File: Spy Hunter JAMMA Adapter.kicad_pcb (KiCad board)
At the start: 2 copper layers, 111.4 x 135.4 mm, 88 parts, among them P1 1K, P2 1K, P3 10K, P4 1K, SW2 SW_DIP_SPSTx02_Slide_9.78x7.2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, U1 74LS86, U10 NE555, U11 LM386, U12 CD4099B, U2 74LS74, U3 74LS00, U4 74LS00, U5 74LS191, U6 74LS191, U7 NE555, U8 74LS157, U9 74LS157

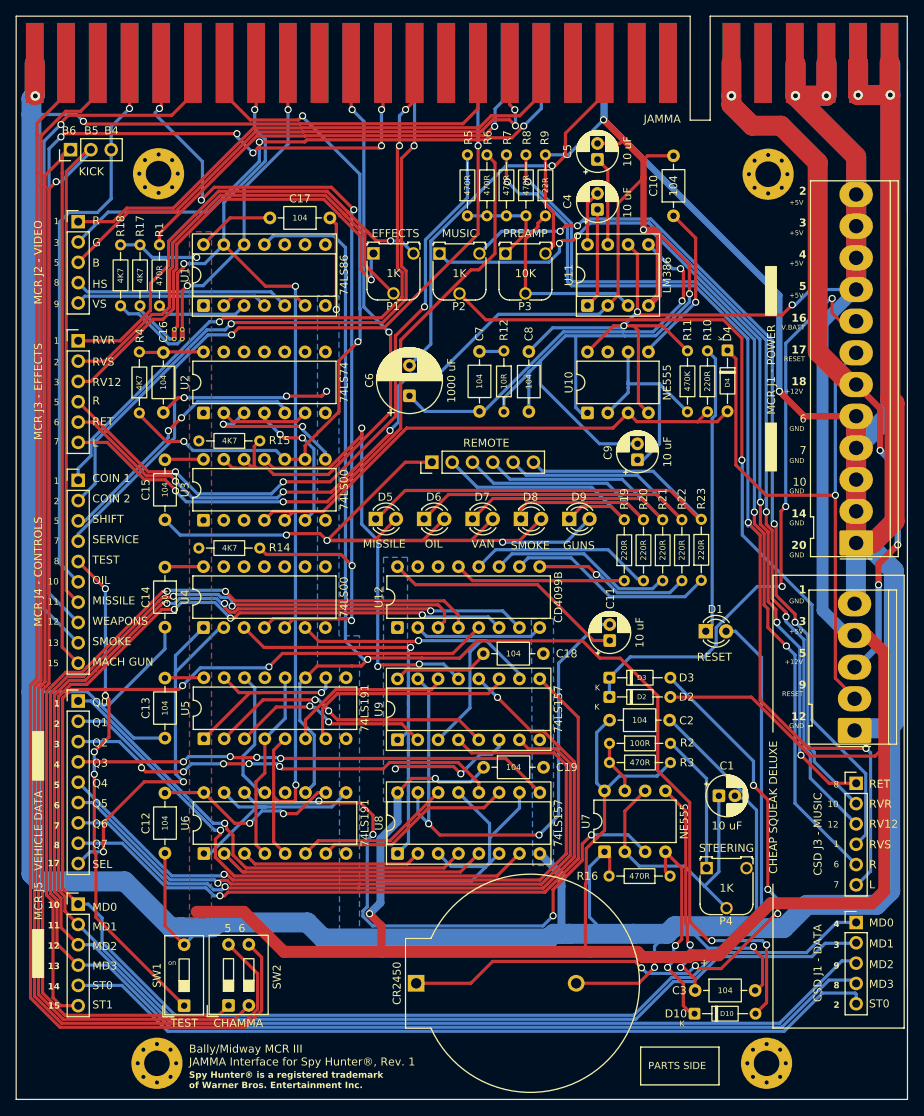
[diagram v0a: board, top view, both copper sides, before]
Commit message: minor cleanup and fine tuning
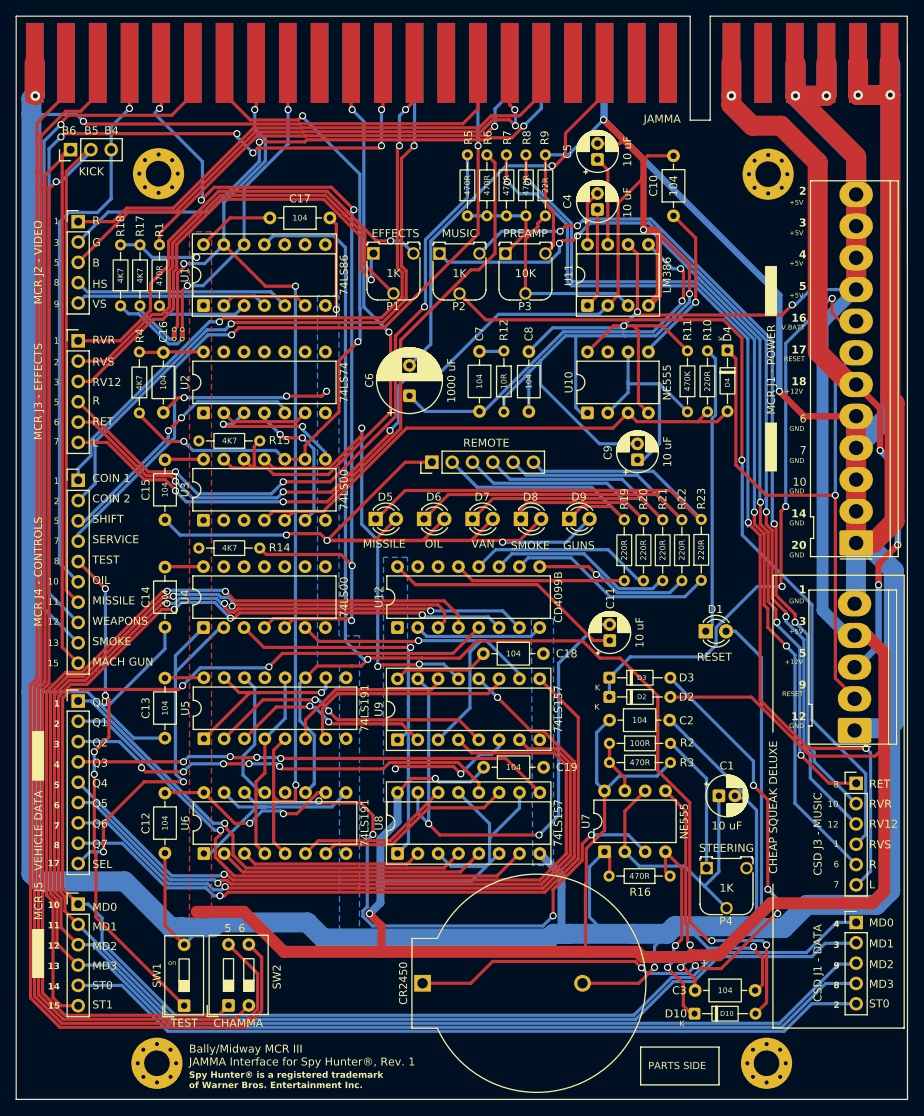
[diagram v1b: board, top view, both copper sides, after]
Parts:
- moved CR2450 0.80 mm to (105.2, 147.4)
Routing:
- net J5_ST0: track 102.9 -> 101.0 mm
- net EFFECTS_RVR: track 57.8 -> 56.6 mm
- net BATT+: track 85.3 -> 84.5 mm
- net GND: track 1352.2 -> 1351.4 mm
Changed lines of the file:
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@@
 		(tags "Resistor Axial_DIN0204 series Axial Horizontal pin pitch 7.62mm 0.167W length 3.6mm diameter 1.6mm")
 		(property "Reference" "R16"
-			(at 10.335 0 0)
+			(at 3.735 -2 0)
 			(layer "F.SilkS")
 			(effects
@@
 	(footprint "Battery:BatteryHolder_ComfortableElectronic_CH273-2450_1x2450"
 		(layer "F.Cu")
-		(at 104.4 147.4)
+		(at 105.2 147.4)
 		(descr "Comfortable Electronic CR2450 battery holder, http://www.comf.com.tw/ProductDetail.asp?no=148")
 		(tags "Comfortable Electronic CR2450")
@@
 	)
 	(segment
+		(start 132.215 147.4)
+		(end 134.2 145.415)
+		(width 0.4)
+		(layer "F.Cu")
+		(net 1)
+	)
+	(segment
 		(start 146.962582 148.297895)
 		(end 146.774846 148.297895)
@@
 	)
 	(segment
-		(start 132.215 147.4)
-		(end 134.2 145.415)
-		(width 0.4)
-		(layer "F.Cu")
-		(net 1)
-	)
-	(segment
 		(start 89.891275 39.983445)
 		(end 63.133445 39.983445)
@@
 	)
 	(segment
-		(start 101.878455 89.359822)
-		(end 99.188277 92.05)
+		(start 125.2 147.4)
+		(end 132.215 147.4)
 		(width 0.4)
 		(layer "F.Cu")
@@
 	)
 	(segment
-		(start 124.4 147.4)
-		(end 132.215 147.4)
+		(start 101.878455 89.359822)
+		(end 99.188277 92.05)
 		(width 0.4)
 		(layer "F.Cu")
@@
 	)
 	(segment
-		(start 99.065 54.224639)
-		(end 98.220181 53.379819)
-		(width 0.4)
-		(layer "F.Cu")
-		(net 7)
-	)
-	(segment
 		(start 76.893889 51.214539)
 		(end 76.88823 51.214539)
@@
 	)
 	(segment
-		(start 131.765 144.665)
-		(end 132.565 145.465)
+		(start 149.384414 138.7)
+		(end 149.592207 138.7)
 		(width 0.4)
 		(layer "F.Cu")
@@
 	)
 	(segment
-		(start 149.384414 138.7)
-		(end 149.592207 138.7)
+		(start 111.23 147.4)
+		(end 113.965 144.665)
 		(width 0.4)
 		(layer "F.Cu")
@@
 	)
 	(segment
-		(start 139.304568 145.193907)
-		(end 139.675661 145.565)
+		(start 131.765 144.665)
+		(end 132.565 145.465)
 		(width 0.4)
 		(layer "F.Cu")
@@
 	)
 	(segment
-		(start 104.4 147.4)
-		(end 111.23 147.4)
+		(start 139.304568 145.193907)
+		(end 139.675661 145.565)
 		(width 0.4)
 		(layer "F.Cu")
@@
 	)
 	(segment
-		(start 111.23 147.4)
-		(end 113.965 144.665)
+		(start 142.519414 145.565)
+		(end 149.384414 138.7)
 		(width 0.4)
 		(layer "F.Cu")
@@
 	)
 	(segment
-		(start 142.519414 145.565)
-		(end 149.384414 138.7)
+		(start 139.675661 145.565)
+		(end 142.519414 145.565)
 		(width 0.4)
 		(layer "F.Cu")
@@
 	)
 	(segment
-		(start 139.675661 145.565)
-		(end 142.519414 145.565)
+		(start 105.2 147.4)
+		(end 111.23 147.4)
 		(width 0.4)
 		(layer "F.Cu")
@@
 	)
 	(segment
-		(start 62.155 142.585)
-		(end 63.987893 142.585)
+		(start 63.987893 142.585)
+		(end 73.802894 152.4)
 		(width 0.4)
 		(layer "B.Cu")
@@
 	)
 	(segment
-		(start 74.84514 99.3)
-		(end 79.44402 99.3)
+		(start 149.83 152.4)
+		(end 157.23 145)
 		(width 0.4)
 		(layer "B.Cu")
@@
 	)
 	(segment
-		(start 63.987893 142.585)
-		(end 73.802894 152.4)
+		(start 74.84514 99.3)
+		(end 79.44402 99.3)
 		(width 0.4)
 		(layer "B.Cu")
@@
 	)
 	(segment
-		(start 159.12 144.6)
-		(end 159.4 144.88)
+		(start 157.23 145)
+		(end 159.28 145)
 		(width 0.4)
 		(layer "B.Cu")
@@
 	)
 	(segment
-		(start 149.83 152.4)
-		(end 157.63 144.6)
+		(start 74.23014 99.915)
+		(end 74.84514 99.3)
 		(width 0.4)
 		(layer "B.Cu")
@@
 	)
 	(segment
-		(start 157.63 144.6)
-		(end 159.12 144.6)
+		(start 73.802894 152.4)
+		(end 149.83 152.4)
 		(width 0.4)
 		(layer "B.Cu")
@@
 	)
 	(segment
-		(start 74.23014 99.915)
-		(end 74.84514 99.3)
+		(start 62.155 142.585)
+		(end 63.987893 142.585)
 		(width 0.4)
 		(layer "B.Cu")
@@
 	)
 	(segment
-		(start 73.802894 152.4)
-		(end 149.83 152.4)
+		(start 159.28 145)
+		(end 159.4 144.88)
 		(width 0.4)
 		(layer "B.Cu")
@@
 	)
 	(segment
-		(start 73.595787 152.9)
-		(end 65.820787 145.125)
+		(start 81.391568 100.258807)
+		(end 81.391568 99.589322)
 		(width 0.4)
 		(layer "B.Cu")
@@
 	)
 	(segment
-		(start 81.391568 100.258807)
-		(end 81.391568 99.589322)
+		(start 159.4 147.42)
+		(end 155.591223 147.42)
 		(width 0.4)
 		(layer "B.Cu")
@@
 	)
 	(segment
-		(start 158.98 147)
-		(end 156.011223 147)
+		(start 73.595787 152.9)
+		(end 65.820787 145.125)
 		(width 0.4)
 		(layer "B.Cu")
@@
 	)
 	(segment
-		(start 159.4 147.42)
-		(end 158.98 147)
+		(start 155.591223 147.42)
+		(end 150.111223 152.9)
 		(width 0.4)
 		(layer "B.Cu")
@@
 	)
 	(segment
-		(start 156.011223 147)
-		(end 150.111223 152.9)
-		(width 0.4)
-		(layer "B.Cu")
-		(net 96)
-	)
-	(segment
 		(start 58.2 110.935987)
 		(end 58.599 110.536987)
@@
 	)
 	(segment
-		(start 159.4 148.76)
-		(end 159.265 148.625)
-		(width 0.4)
-		(layer "B.Cu")
-		(net 100)
-	)
-	(segment
 		(start 73.358418 153.4)
 		(end 67.623418 147.665)
@@
 	)
 	(segment
-		(start 155.175 148.625)
+		(start 153.84 149.96)
 		(end 150.4 153.4)
 		(width 0.4)
@@
 	)
 	(segment
-		(start 159.4 149.96)
-		(end 159.4 148.76)
-		(width 0.4)
-		(layer "B.Cu")
-		(net 100)
-	)
-	(segment
 		(start 67.623418 147.665)
 		(end 62.155 147.665)
@@
 	)
 	(segment
-		(start 159.265 148.625)
-		(end 155.175 148.625)
+		(start 159.4 149.96)
+		(end 153.84 149.96)
 		(width 0.4)
 		(layer "B.Cu")
